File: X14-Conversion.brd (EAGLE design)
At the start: 50.8 x 68.6 mm, 25 parts, among them P1 282837-2, P2 282837-2, P3 282837-2, U1 BUCK,LM2678S-ADJ

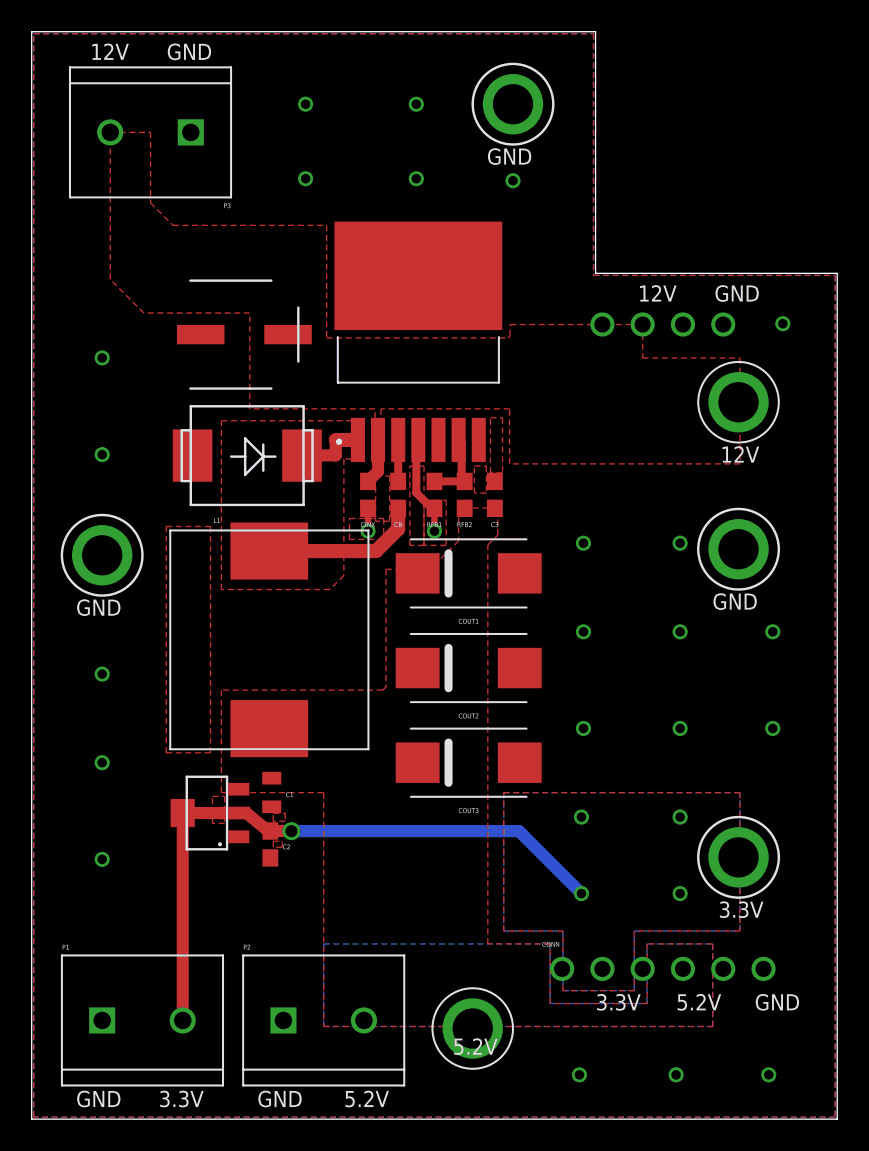
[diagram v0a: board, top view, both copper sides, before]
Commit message: fix board
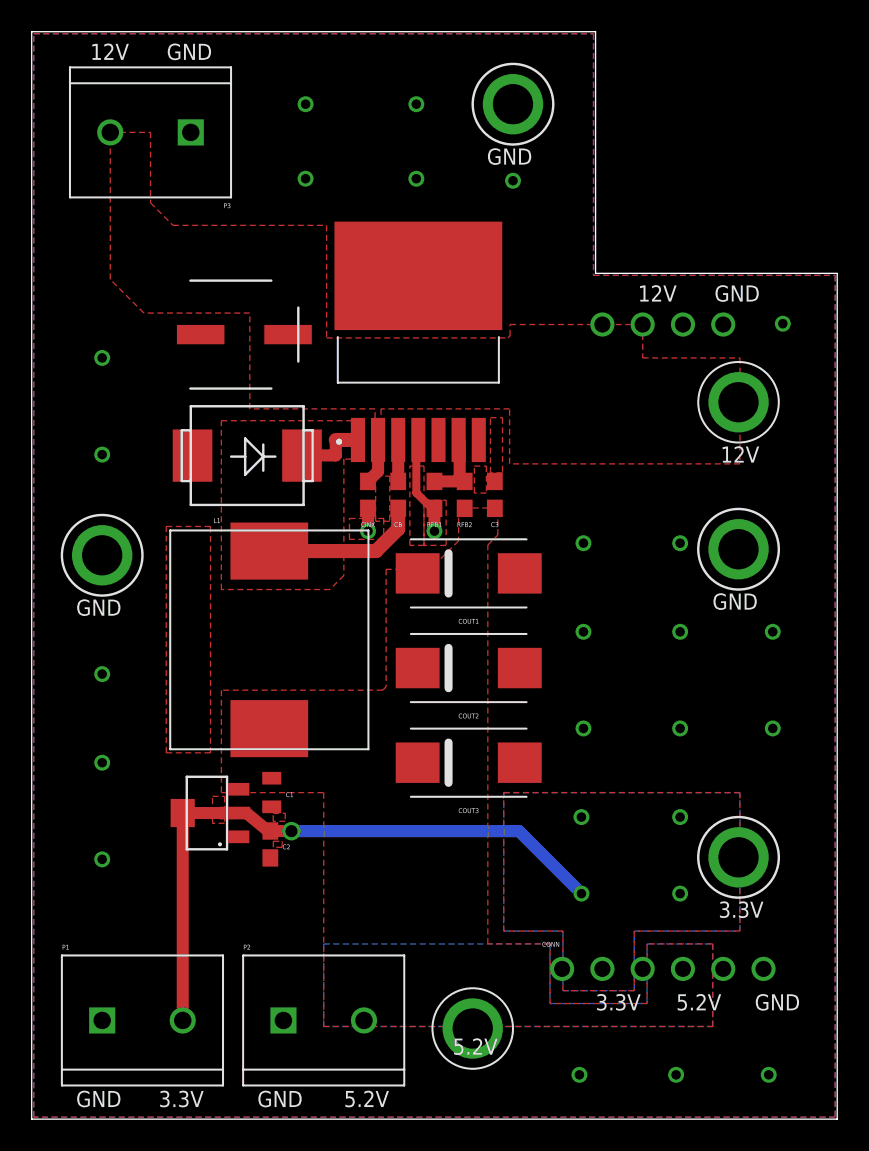
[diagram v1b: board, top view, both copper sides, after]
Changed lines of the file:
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@@
 </class>
 </classes>
-<designrules name="ECE_Senior_Design">
+<designrules name="477">
 <description language="de">&lt;b&gt;EAGLE Design Rules&lt;/b&gt;
 &lt;p&gt;
@@
 Einstellungen hier und speichern die Design Rules unter
 einem neuen Namen ab.</description>
-<description language="en">&lt;b&gt;ECE 402/477 Design Rules Version 2&lt;/b&gt;
+<description language="en">description[de] = &lt;b&gt;EAGLE Design Rules&lt;/b&gt;
+&lt;p&gt;
+Die Standard-Design-Rules sind so gewÃ¤hlt, dass sie fÃ¼r
+die meisten Anwendungen passen. Sollte ihre Platine
+besondere Anforderungen haben, treffen Sie die erforderlichen
+Einstellungen hier und speichern die Design Rules unter
+einem neuen Namen ab.
+description[en] = &lt;b&gt;ECE 402/477 Design Rules Version 2&lt;/b&gt;
 &lt;p&gt;
 These are the design rules to use for Purdue University electrical and computer engineering senior design PCBs.
@@
 Please make sure your boards conform to these design rules.
 &lt;/p&gt;
+layerSetup = (1*16)
+mtCopper = 0.0356mm 0.0356mm 0.0356mm 0.0356mm 0.0356mm 0.0356mm 0.0356mm 0.0356mm 0.0356mm 0.0356mm 0.0356mm 0.0356mm 0.0356mm 0.0356mm 0.0356mm 0.0356mm
+mtIsolate = 1.5011mm 0.1499mm 0.2007mm 0.1499mm 0.2007mm 0.1499mm 0.2007mm 0.1499mm 0.2007mm 0.1499mm 0.2007mm 0.1499mm 0.2007mm 0.1499mm 0.2007mm
+mdWireWire = 8mil
+mdWirePad = 8mil
+mdWireVia = 8mil
+mdPadPad = 6mil
+mdPadVia = 8mil
+mdViaVia = 8mil
+mdSmdPad = 6mil
+mdSmdVia = 6mil
+mdSmdSmd = 6mil
+mdViaViaSameLayer = 8mil
+mnLayersViaInSmd = 2
+mdCopperDimension = 15mil
+mdDrill = 8mil
+mdSmdStop = 0mil
+msWidth = 8mil
+msDrill = 13mil
+msMicroVia = 13mil
+msBlindViaRatio = 0.500000
+rvPadTop = 0.250000
+rvPadInner = 0.250000
+rvPadBottom = 0.250000
+rvViaOuter = 0.250000
+rvViaInner = 0.250000
+rvMicroViaOuter = 0.250000
+rvMicroViaInner = 0.250000
+rlMinPadTop = 7mil
+rlMaxPadTop = 20mil
+rlMinPadInner = 7mil
+rlMaxPadInner = 20mil
+rlMinPadBottom = 7mil
+rlMaxPadBottom = 20mil
+rlMinViaOuter = 7mil
+rlMaxViaOuter = 20mil
+rlMinViaInner = 7mil
+rlMaxViaInner = 20mil
+rlMinMicroViaOuter = 4mil
+rlMaxMicroViaOuter = 20mil
+rlMinMicroViaInner = 4mil
+rlMaxMicroViaInner = 20mil
+psTop = -1
+psBottom = -1
+psFirst = -1
+psElongationLong = 100
+psElongationOffset = 100
+mvStopFrame = 1.000000
+mvCreamFrame = 0.000000
+mlMinStopFrame = 3mil
+mlMaxStopFrame = 3mil
+mlMinCreamFrame = 0mil
+mlMaxCreamFrame = 0mil
+mlViaStopLimit = 0mil
+srRoundness = 0.000000
+srMinRoundness = 0mil
+srMaxRoundness = 0mil
+slThermalIsolate = 10mil
+slThermalsForVias = 0
+dpMaxLengthDifference = 10mm
+dpGapFactor = 2.500000
+checkGrid = 0
+checkAngle = 0
+checkFont = 1
+checkRestrict = 1
+useDiameter = 13
+maxErrors = 50
 </description>
 <param name="layerSetup" value="(1*16)"/>
-<param name="mtCopper" value="0.0356mm 0.0356mm 0.0356mm 0.0356mm 0.0356mm 0.0356mm 0.0356mm 0.0356mm 0.0356mm 0.0356mm 0.0356mm 0.0356mm 0.0356mm 0.0356mm 0.0356mm 0.0356mm"/>
-<param name="mtIsolate" value="1.5011mm 0.1499mm 0.2007mm 0.1499mm 0.2007mm 0.1499mm 0.2007mm 0.1499mm 0.2007mm 0.1499mm 0.2007mm 0.1499mm 0.2007mm 0.1499mm 0.2007mm"/>
-<param name="mdWireWire" value="8mil"/>
-<param name="mdWirePad" value="8mil"/>
-<param name="mdWireVia" value="8mil"/>
+<param name="mtCopper" value="0.035mm 0.035mm 0.035mm 0.035mm 0.035mm 0.035mm 0.035mm 0.035mm 0.035mm 0.035mm 0.035mm 0.035mm 0.035mm 0.035mm 0.035mm 0.035mm"/>
+<param name="mtIsolate" value="1.5mm 0.15mm 0.2mm 0.15mm 0.2mm 0.15mm 0.2mm 0.15mm 0.2mm 0.15mm 0.2mm 0.15mm 0.2mm 0.15mm 0.2mm"/>
+<param name="mdWireWire" value="6mil"/>
+<param name="mdWirePad" value="6mil"/>
+<param name="mdWireVia" value="6mil"/>
 <param name="mdPadPad" value="6mil"/>
-<param name="mdPadVia" value="8mil"/>
-<param name="mdViaVia" value="8mil"/>
+<param name="mdPadVia" value="6mil"/>
+<param name="mdViaVia" value="6mil"/>
 <param name="mdSmdPad" value="6mil"/>
 <param name="mdSmdVia" value="6mil"/>
 <param name="mdSmdSmd" value="6mil"/>
-<param name="mdViaViaSameLayer" value="8mil"/>
+<param name="mdViaViaSameLayer" value="6mil"/>
 <param name="mnLayersViaInSmd" value="2"/>
-<param name="mdCopperDimension" value="15mil"/>
-<param name="mdDrill" value="8mil"/>
+<param name="mdCopperDimension" value="40mil"/>
+<param name="mdDrill" value="6mil"/>
 <param name="mdSmdStop" value="0mil"/>
-<param name="msWidth" value="8mil"/>
-<param name="msDrill" value="13mil"/>
-<param name="msMicroVia" value="13mil"/>
+<param name="msWidth" value="6mil"/>
+<param name="msDrill" value="0.35mm"/>
+<param name="msMicroVia" value="9.99mm"/>
 <param name="msBlindViaRatio" value="0.5"/>
 <param name="rvPadTop" value="0.25"/>
@@
 <param name="rvMicroViaOuter" value="0.25"/>
 <param name="rvMicroViaInner" value="0.25"/>
-<param name="rlMinPadTop" value="7mil"/>
+<param name="rlMinPadTop" value="10mil"/>
 <param name="rlMaxPadTop" value="20mil"/>
-<param name="rlMinPadInner" value="7mil"/>
+<param name="rlMinPadInner" value="10mil"/>
 <param name="rlMaxPadInner" value="20mil"/>
-<param name="rlMinPadBottom" value="7mil"/>
+<param name="rlMinPadBottom" value="10mil"/>
 <param name="rlMaxPadBottom" value="20mil"/>
-<param name="rlMinViaOuter" value="7mil"/>
+<param name="rlMinViaOuter" value="8mil"/>
 <param name="rlMaxViaOuter" value="20mil"/>
-<param name="rlMinViaInner" value="7mil"/>
+<param name="rlMinViaInner" value="8mil"/>
 <param name="rlMaxViaInner" value="20mil"/>
 <param name="rlMinMicroViaOuter" value="4mil"/>
@@
 <param name="mvStopFrame" value="1"/>
 <param name="mvCreamFrame" value="0"/>
-<param name="mlMinStopFrame" value="3mil"/>
-<param name="mlMaxStopFrame" value="3mil"/>
+<param name="mlMinStopFrame" value="4mil"/>
+<param name="mlMaxStopFrame" value="4mil"/>
 <param name="mlMinCreamFrame" value="0mil"/>
 <param name="mlMaxCreamFrame" value="0mil"/>
@@
 <via x="4.445" y="16.383" extent="1-16" drill="0.6"/>
 <wire x1="25.4" y1="38.52" x2="25.4" y2="38.354" width="0.4064" layer="1"/>
-<wire x1="25.4" y1="38.354" x2="25.4" y2="37.084" width="0.4064" layer="1"/>
+<wire x1="25.4" y1="38.354" x2="25.4" y2="37.084" width="0.762" layer="1"/>
 <via x="25.4" y="37.084" extent="1-16" drill="0.6"/>
-<wire x1="21.209" y1="38.52" x2="21.209" y2="37.084" width="0.4064" layer="1"/>
+<wire x1="21.209" y1="38.52" x2="21.209" y2="37.084" width="0.762" layer="1"/>
 <via x="21.209" y="37.084" extent="1-16" drill="0.6"/>
 <wire x1="24.384" y1="42.832" x2="24.257" y2="42.705" width="0.508" layer="1"/>
@@
 <contactref element="CB" pad="1"/>
 <contactref element="U1" pad="3"/>
-<wire x1="23.114" y1="42.832" x2="23.114" y2="40.22" width="0.508" layer="1"/>
+<wire x1="23.114" y1="42.832" x2="23.114" y2="40.22" width="0.762" layer="1"/>
 </signal>
 <signal name="FB">
@@
 <contactref element="RFB2" pad="1"/>
 <contactref element="U1" pad="6"/>
-<wire x1="25.4" y1="40.22" x2="27.305" y2="40.22" width="0.508" layer="1"/>
-<wire x1="26.924" y1="42.832" x2="27.11576875" y2="42.64023125" width="0.508" layer="1"/>
-<wire x1="27.305" y1="40.22" x2="27.11576875" y2="40.40923125" width="0.508" layer="1"/>
-<wire x1="27.11576875" y1="42.64023125" x2="27.11576875" y2="40.40923125" width="0.508" layer="1"/>
+<wire x1="25.4" y1="40.22" x2="27.305" y2="40.22" width="0.762" layer="1"/>
+<wire x1="26.924" y1="42.832" x2="26.98876875" y2="42.76723125" width="0.508" layer="1"/>
+<wire x1="27.305" y1="40.22" x2="26.98876875" y2="40.53623125" width="0.508" layer="1"/>
+<wire x1="26.98876875" y1="42.76723125" x2="26.98876875" y2="40.53623125" width="0.762" layer="1"/>
 </signal>
 <signal name="CUTOUT5">
